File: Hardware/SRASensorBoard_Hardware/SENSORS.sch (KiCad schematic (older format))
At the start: 85 parts, among them J1 USB_A, Q1 BSS138, Q10 BSS138, Q11 BSS138, Q12 BSS138, Q13 BSS138, Q2 BSS138, Q3 BSS138, Q4 BSS138, Q5 BSS138, Q6 BSS138, Q9 BSS138, U3 FT230XS

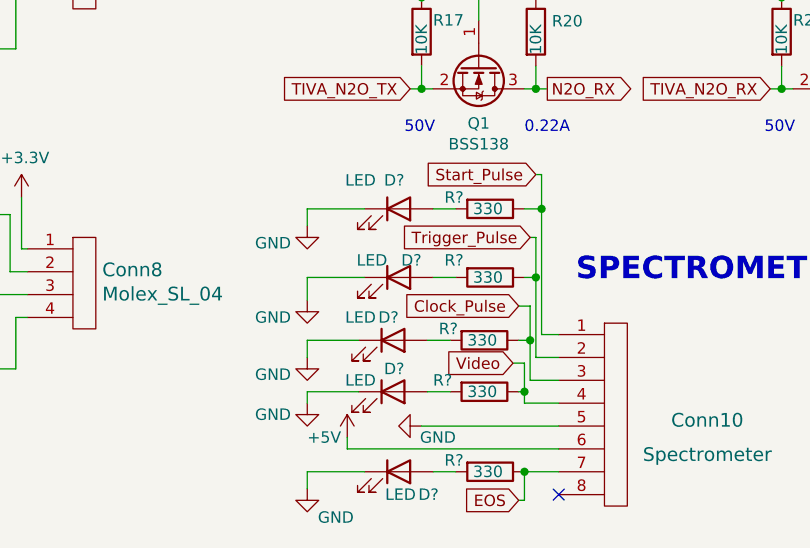
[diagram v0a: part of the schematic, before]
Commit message: Board Progress 7 (final rev 1)
Final edits for REV 1
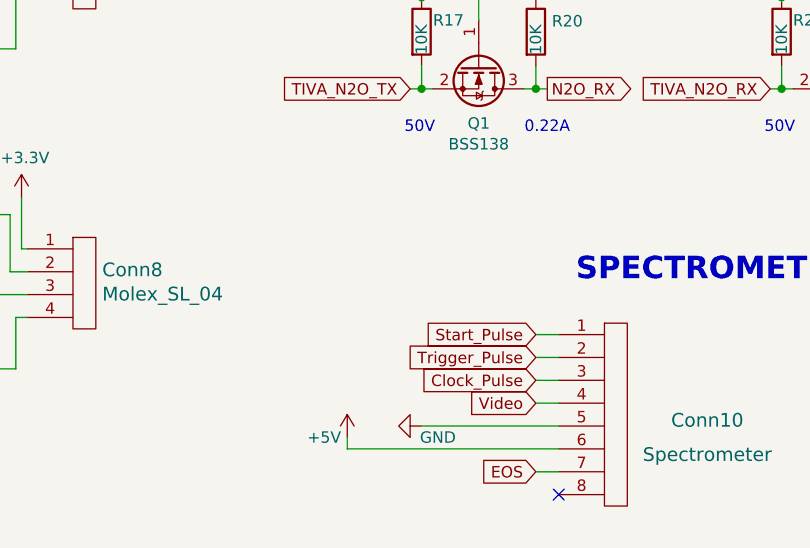
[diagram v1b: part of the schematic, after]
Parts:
- removed D? (x5): LED, Diode_SMD:D_0603_1608Metric_Pad1.05x0.95mm_HandSolder, symbol Device:LED
- removed R? (x5): 330, Resistor_SMD:R_0603_1608Metric_Pad1.05x0.95mm_HandSolder, symbol Device:R
- C8: footprint Capacitor_THT:CP_Radial_D12.5mm_P5.00mm -> Capacitor_THT:CP_Radial_D5.0mm_P2.50mm
